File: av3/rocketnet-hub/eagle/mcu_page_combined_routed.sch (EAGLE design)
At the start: 443 parts, among them J1 ROCKETNET-CONNECTOR-16M, J10 UART Header, J11 I2C Header, J12 BOOT1 Jumper, J13 PGOOD Jumper, J14 ROCKETNET-UMBILICAL-18, J15 Auxiliary Header, J16 Auxiliary Header, J17 Auxiliary Header, J18 Auxiliary Header, J19 Auxiliary Header, J2 ROCKETNET-CONNECTOR-16M, J20 Auxiliary Header, J21 Auxiliary Header, J22 Debug Header, J3 ROCKETNET-CONNECTOR-16M, J4 ROCKETNET-CONNECTOR-16M, J5 BOOT0 Jumper, J6 ROCKETNET-CONNECTOR-16M, J7 ROCKETNET-CONNECTOR-16M, J8 ROCKETNET-CONNECTOR-16M, J9 ROCKETNET-BATTERY-14, Q1 NTR401P, Q2 FDS6680ASOIC8, Q3 FDS6680ASOIC8, Q4 FDS6680ASOIC8, Q5 SIS412DNSOP-8, Q6 BSS138W-7-F, Q7 SIS412DNSOP-8, Q8 PMV45EN, Q9 NTR4101P, T10 ALT4532, T11 ALT4532, T12 ALT4532, T13 ALT4532, T14 ALT4532, T15 ALT4532, T16 ALT4532, T17 ALT4532, T18 ALT4532, T20 NDS335N, T3 ALT4532, T4 ALT4532, T5 ALT4532, T6 ALT4532, T7 ALT4532, T8 ALT4532, T9 ALT4532, U1 STM32F407V100-PIN_QFP, U10 TPS2420QFN-16, U11 TPS2420QFN-16, U12 TPS2420QFN-16, U13 TPS2420QFN-16, U14 MAX4734ETC+, U15 MAX4734ETC+, U2 BQ24725QFN-20, U3 SN65220DBV, U4 KS8999, U5 LTM8023, U6 MIC37101-2.1YM, U7 TPS2420QFN-16, U8 TPS2420QFN-16, U9 TPS2420QFN-16

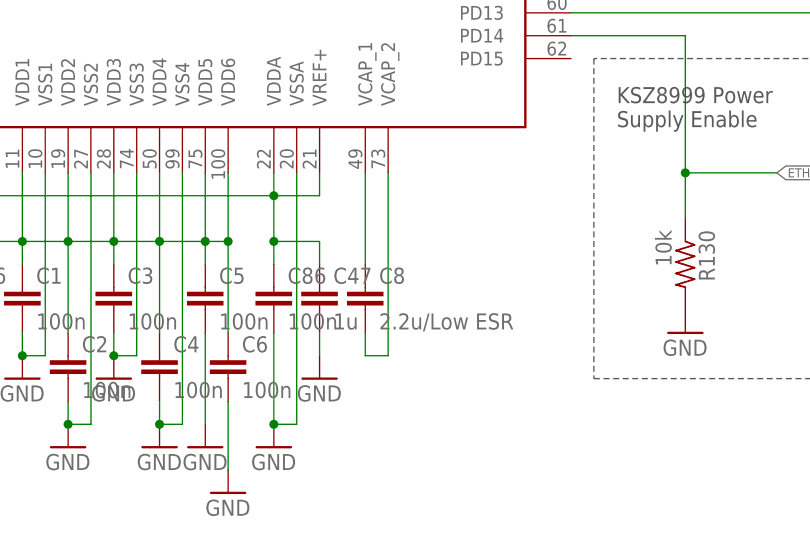
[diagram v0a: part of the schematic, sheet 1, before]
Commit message: Clean up of decoupling caps and feeds around STM32. Fixed mistake in VCAP1/VCAP2 capacitors.
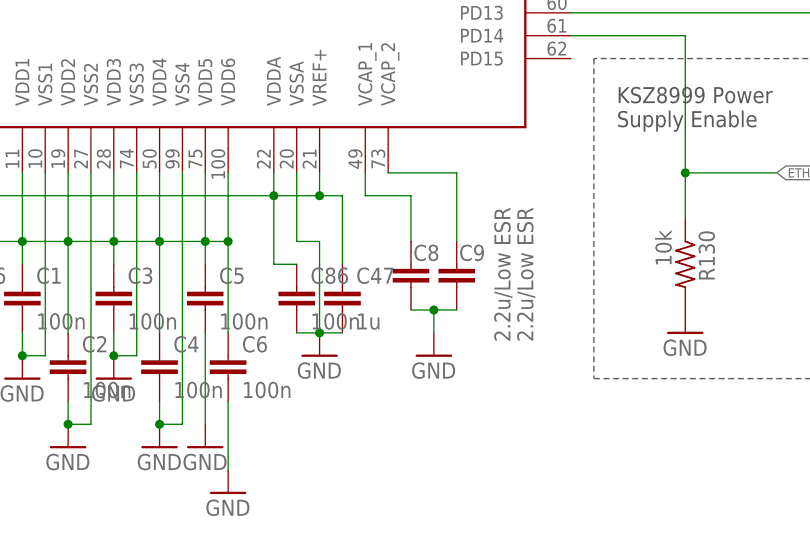
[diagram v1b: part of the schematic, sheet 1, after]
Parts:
- added C9: 2.2u/Low ESR, rcl_custom:C-EU0402-B-NOSILK
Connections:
- net GND: now also C8.2, C9.2
- net N$167: now also C9.1; no longer C8.2
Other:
- moved on the sheet: C47, C8, C86
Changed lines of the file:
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@@
 <setting verticaltext="up"/>
 </settings>
-<grid distance="0.1" unitdist="inch" unit="inch" style="lines" multiple="1" display="no" altdistance="0.01" altunitdist="inch" altunit="inch"/>
+<grid distance="0.05" unitdist="inch" unit="inch" style="lines" multiple="2" display="no" altdistance="0.01" altunitdist="inch" altunit="inch"/>
 <layers>
 <layer number="1" name="Top" color="4" fill="1" visible="no" active="no"/>
@@
 <part name="R48" library="rcl_custom" deviceset="R-US_" device="0402-B-NOSILK" value="1.2k"/>
 <part name="C86" library="rcl_custom" deviceset="C-EU" device="0402-B-NOSILK" value="100n"/>
-<part name="GND17" library="supply1" deviceset="GND" device=""/>
 <part name="GND18" library="supply1" deviceset="GND" device=""/>
 <part name="GND19" library="supply1" deviceset="GND" device=""/>
@@
 <part name="GND81" library="supply1" deviceset="GND" device=""/>
 <part name="C47" library="rcl_custom" deviceset="C-EU" device="0603-B-NOSILK" value="1u"/>
-<part name="GND94" library="supply1" deviceset="GND" device=""/>
 <part name="OFF_ROCKET_CONNECTORS" library="frames" deviceset="FRAME_A_L" device="" value="Off Rocket Connectors"/>
 <part name="GND91" library="supply1" deviceset="GND" device=""/>
@@
 <part name="GND150" library="supply1" deviceset="GND" device=""/>
 <part name="GND152" library="supply1" deviceset="GND" device=""/>
+<part name="C9" library="rcl_custom" deviceset="C-EU" device="0402-B-NOSILK" value="2.2u/Low ESR"/>
+<part name="GND151" library="supply1" deviceset="GND" device=""/>
+<part name="GND153" library="supply1" deviceset="GND" device=""/>
 </parts>
 <sheets>
@@
 <instance part="C5" gate="CE" x="111.76" y="314.96"/>
 <instance part="C6" gate="CE" x="114.3" y="307.34"/>
-<instance part="C8" gate="CE" x="129.54" y="314.96"/>
+<instance part="C8" gate="CE" x="134.62" y="317.5" smashed="yes">
+<attribute name="NAME" x="134.874" y="317.881" size="1.778" layer="95"/>
+<attribute name="VALUE" x="148.209" y="308.864" size="1.778" layer="96" rot="R90"/>
+</instance>
 <instance part="GND2" gate="1" x="96.52" y="297.18"/>
 <instance part="GND3" gate="1" x="101.6" y="304.8"/>
@@
 <instance part="+3V7" gate="G$1" x="213.36" y="358.14"/>
 <instance part="E5" gate="E" x="83.82" y="325.12"/>
-<instance part="C86" gate="CE" x="119.38" y="314.96"/>
-<instance part="GND17" gate="1" x="119.38" y="297.18"/>
+<instance part="C86" gate="CE" x="121.92" y="314.96"/>
 <instance part="R15" gate="R" x="12.7" y="370.84" rot="R270"/>
 <instance part="R17" gate="R" x="5.08" y="370.84" rot="R270"/>
@@
 <instance part="C46" gate="CE" x="83.82" y="314.96"/>
 <instance part="GND81" gate="1" x="83.82" y="304.8"/>
-<instance part="C47" gate="CE" x="124.46" y="314.96"/>
-<instance part="GND94" gate="1" x="124.46" y="304.8"/>
+<instance part="C47" gate="CE" x="127" y="314.96"/>
 <instance part="R130" gate="R" x="165.1" y="317.5" smashed="yes" rot="R270">
 <attribute name="NAME" x="166.5986" y="321.31" size="1.778" layer="95" rot="R270"/>
@@
 <instance part="GND8" gate="1" x="-5.08" y="350.52"/>
 <instance part="R25" gate="R" x="182.88" y="414.02" rot="R180"/>
+<instance part="C9" gate="CE" x="139.7" y="317.5" smashed="yes">
+<attribute name="NAME" x="139.954" y="317.881" size="1.778" layer="95"/>
+<attribute name="VALUE" x="145.669" y="308.864" size="1.778" layer="96" rot="R90"/>
+</instance>
+<instance part="GND151" gate="1" x="137.16" y="307.34"/>
+<instance part="GND153" gate="1" x="124.46" y="307.34"/>
 </instances>
 <busses>
@@
 <pinref part="C8" gate="CE" pin="1"/>
 <pinref part="U1" gate="U1" pin="VCAP_1"/>
-<wire x1="129.54" y1="317.5" x2="129.54" y2="327.66" width="0.1524" layer="91"/>
+<wire x1="134.62" y1="320.04" x2="134.62" y2="325.12" width="0.1524" layer="91"/>
+<wire x1="134.62" y1="325.12" x2="129.54" y2="325.12" width="0.1524" layer="91"/>
+<wire x1="129.54" y1="325.12" x2="129.54" y2="327.66" width="0.1524" layer="91"/>
 </segment>
 </net>
@@
 </segment>
 <segment>
-<pinref part="GND17" gate="1" pin="GND"/>
+<pinref part="U1" gate="U1" pin="VSSA"/>
+<wire x1="121.92" y1="327.66" x2="121.92" y2="320.04" width="0.1524" layer="91"/>
+<wire x1="121.92" y1="320.04" x2="124.46" y2="320.04" width="0.1524" layer="91"/>
+<wire x1="124.46" y1="320.04" x2="124.46" y2="317.5" width="0.1524" layer="91"/>
+<wire x1="124.46" y1="317.5" x2="124.46" y2="309.88" width="0.1524" layer="91"/>
+<pinref part="GND153" gate="1" pin="GND"/>
 <pinref part="C86" gate="CE" pin="2"/>
-<wire x1="119.38" y1="299.72" x2="119.38" y2="309.88" width="0.1524" layer="91"/>
-<pinref part="U1" gate="U1" pin="VSSA"/>
-<wire x1="121.92" y1="327.66" x2="121.92" y2="299.72" width="0.1524" layer="91"/>
-<wire x1="121.92" y1="299.72" x2="119.38" y2="299.72" width="0.1524" layer="91"/>
-<junction x="119.38" y="299.72"/>
+<pinref part="C47" gate="CE" pin="2"/>
+<wire x1="121.92" y1="309.88" x2="124.46" y2="309.88" width="0.1524" layer="91"/>
+<junction x="124.46" y="309.88"/>
+<wire x1="124.46" y1="309.88" x2="127" y2="309.88" width="0.1524" layer="91"/>
 </segment>
 <segment>
@@
 </segment>
 <segment>
-<pinref part="C47" gate="CE" pin="2"/>
-<wire x1="124.46" y1="309.88" x2="124.46" y2="307.34" width="0.1524" layer="91"/>
-<pinref part="GND94" gate="1" pin="GND"/>
-</segment>
-<segment>
 <pinref part="R130" gate="R" pin="2"/>
 <pinref part="GND54" gate="1" pin="GND"/>
@@
 <wire x1="-5.08" y1="358.14" x2="-5.08" y2="353.06" width="0.1524" layer="91"/>
 <pinref part="GND8" gate="1" pin="GND"/>
+</segment>
+<segment>
+<pinref part="C8" gate="CE" pin="2"/>
+<pinref part="C9" gate="CE" pin="2"/>
+<wire x1="134.62" y1="312.42" x2="137.16" y2="312.42" width="0.1524" layer="91"/>
+<pinref part="GND151" gate="1" pin="GND"/>
+<wire x1="137.16" y1="312.42" x2="139.7" y2="312.42" width="0.1524" layer="91"/>
+<wire x1="137.16" y1="312.42" x2="137.16" y2="309.88" width="0.1524" layer="91"/>
+<junction x="137.16" y="312.42"/>
 </segment>
 </net>
@@
 <wire x1="119.38" y1="325.12" x2="119.38" y2="327.66" width="0.1524" layer="91"/>
 <pinref part="C86" gate="CE" pin="1"/>
-<wire x1="119.38" y1="317.5" x2="119.38" y2="320.04" width="0.1524" layer="91"/>
 <junction x="119.38" y="325.12"/>
 <pinref part="U1" gate="U1" pin="VREF+"/>
-<wire x1="119.38" y1="320.04" x2="119.38" y2="325.12" width="0.1524" layer="91"/>
+<wire x1="121.92" y1="317.5" x2="119.38" y2="317.5" width="0.1524" layer="91"/>
+<wire x1="119.38" y1="317.5" x2="119.38" y2="325.12" width="0.1524" layer="91"/>
 <wire x1="119.38" y1="325.12" x2="124.46" y2="325.12" width="0.1524" layer="91"/>
 <wire x1="124.46" y1="325.12" x2="124.46" y2="327.66" width="0.1524" layer="91"/>
 <pinref part="C47" gate="CE" pin="1"/>
-<wire x1="124.46" y1="317.5" x2="124.46" y2="320.04" width="0.1524" layer="91"/>
-<wire x1="124.46" y1="320.04" x2="119.38" y2="320.04" width="0.1524" layer="91"/>
-<junction x="119.38" y="320.04"/>
+<wire x1="127" y1="317.5" x2="127" y2="325.12" width="0.1524" layer="91"/>
+<wire x1="127" y1="325.12" x2="124.46" y2="325.12" width="0.1524" layer="91"/>
+<junction x="124.46" y="325.12"/>
 </segment>
 </net>
@@
 </segment>
 </net>
-<net name="N$167" class="1">
-<segment>
-<pinref part="C8" gate="CE" pin="2"/>
-<wire x1="129.54" y1="307.34" x2="129.54" y2="309.88" width="0.1524" layer="91"/>
-<pinref part="U1" gate="U1" pin="VCAP_2"/>
-<wire x1="129.54" y1="307.34" x2="132.08" y2="307.34" width="0.1524" layer="91"/>
-<wire x1="132.08" y1="307.34" x2="132.08" y2="327.66" width="0.1524" layer="91"/>
-</segment>
-</net>
 <net name="25MHZ_REF_CLK_KSZ" class="0">
 <segment>
@@
 </segment>
 </net>
+<net name="N$167" class="0">
+<segment>
+<pinref part="U1" gate="U1" pin="VCAP_2"/>
+<pinref part="C9" gate="CE" pin="1"/>
+<wire x1="132.08" y1="327.66" x2="139.7" y2="327.66" width="0.1524" layer="91"/>
+<wire x1="139.7" y1="327.66" x2="139.7" y2="320.04" width="0.1524" layer="91"/>
+</segment>
+</net>
